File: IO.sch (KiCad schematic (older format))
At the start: 7 parts

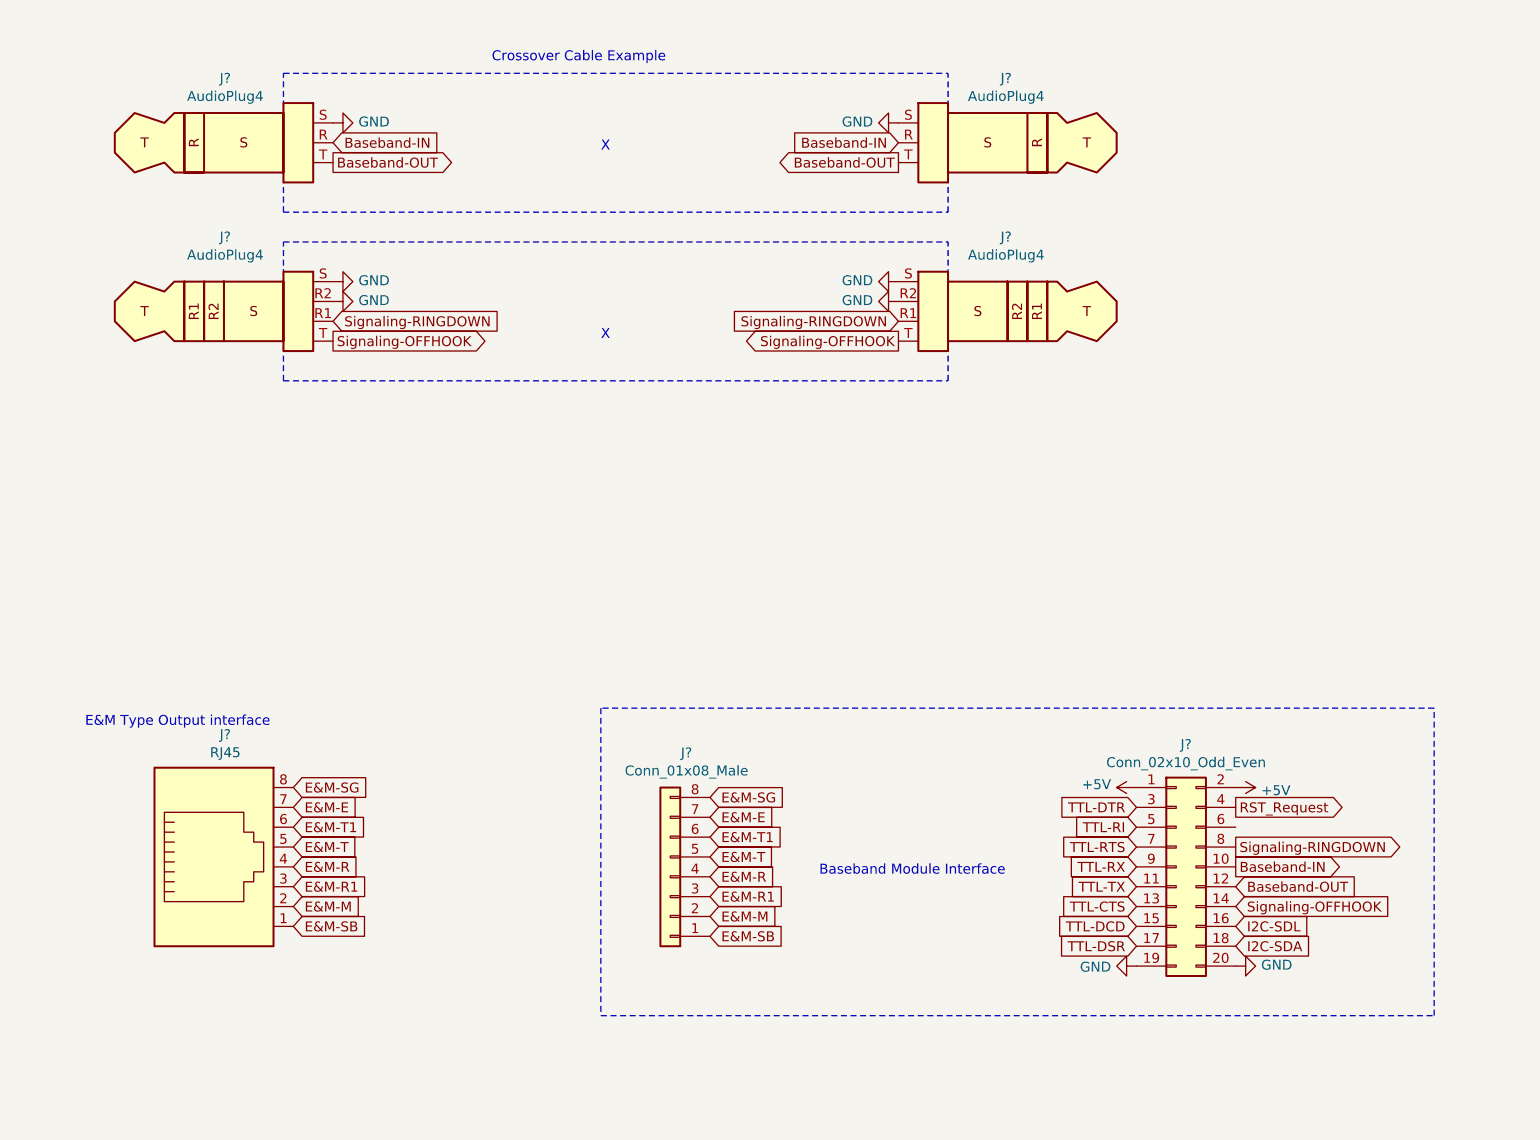
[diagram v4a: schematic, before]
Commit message: io interface updates
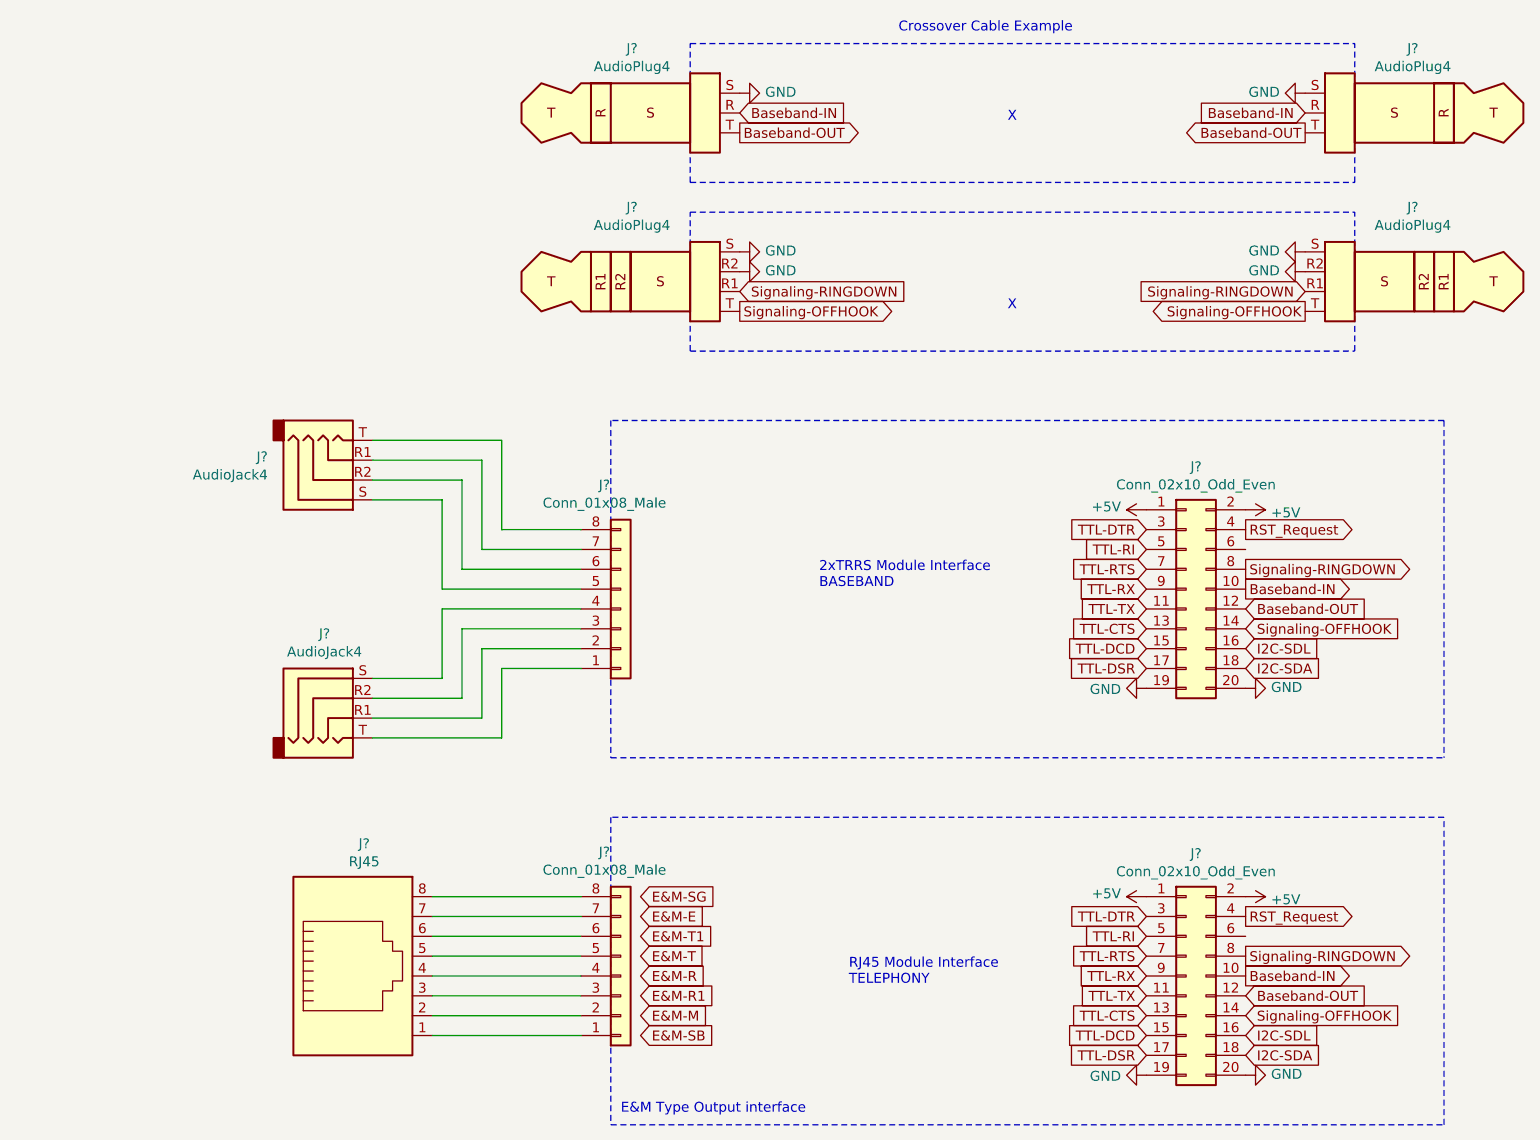
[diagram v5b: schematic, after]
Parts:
- added J?: Conn_01x08_Male, symbol Connector_Generic:Conn_01x08
- added J?: Conn_02x10_Odd_Even, symbol Connector_Generic:Conn_02x10_Odd_Even
- added J? (x2): AudioJack4, symbol Connector:AudioJack4
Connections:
- net +5V: now also J?.1 (Pin_1), J?.2 (Pin_2)
- net Baseband-IN: now also J?.10 (Pin_10)
- net Baseband-OUT: now also J?.12 (Pin_12)
- net E&M-E: no longer J?.7, J?.7 (Pin_7)
- net E&M-M: no longer J?.2, J?.2 (Pin_2)
- net E&M-R: no longer J?.4, J?.4 (Pin_4)
- net E&M-R1: no longer J?.3, J?.3 (Pin_3)
- net E&M-SB: no longer J?.1, J?.1 (Pin_1)
- net E&M-SG: no longer J?.8, J?.8 (Pin_8)
- net E&M-T: no longer J?.5, J?.5 (Pin_5)
- net E&M-T1: no longer J?.6, J?.6 (Pin_6)
- net GND: now also J?.19 (Pin_19), J?.20 (Pin_20)
- net I2C-SDA: now also J?.18 (Pin_18)
- net I2C-SDL: now also J?.16 (Pin_16)
- net RST_Request: now also J?.4 (Pin_4)
- net Signaling-OFFHOOK: now also J?.14 (Pin_14)
- net Signaling-RINGDOWN: now also J?.8 (Pin_8)
- net TTL-CTS: now also J?.13 (Pin_13)
- net TTL-DCD: now also J?.15 (Pin_15)
- net TTL-DSR: now also J?.17 (Pin_17)
- net TTL-DTR: now also J?.3 (Pin_3)
- net TTL-RI: now also J?.5 (Pin_5)
- net TTL-RTS: now also J?.7 (Pin_7)
- net TTL-RX: now also J?.9 (Pin_9)
- net TTL-TX: now also J?.11 (Pin_11)
- new net: J?.1, J?.1 (Pin_1)
- new net: J?.2, J?.2 (Pin_2)
- new net: J?.3, J?.3 (Pin_3)
- new net: J?.4, J?.4 (Pin_4)
- new net: J?.5, J?.5 (Pin_5)
- new net: J?.6, J?.6 (Pin_6)
- new net: J?.7, J?.7 (Pin_7)
- new net: J?.8, J?.8 (Pin_8)
- new net: J?.1 (Pin_1), J?.T
- new net: J?.2 (Pin_2), J?.R1
- new net: J?.3 (Pin_3), J?.R2
- new net: J?.4 (Pin_4), J?.S
- new net: J?.5 (Pin_5), J?.S
- new net: J?.6 (Pin_6), J?.R2
- new net: J?.7 (Pin_7), J?.R1
- new net: J?.8 (Pin_8), J?.T
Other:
- note added: "2xTRRS Module Interface\nBASEBAND"
- note added: "RJ45 Module Interface\nTELEPHONY"
- note removed: "Baseband Module Interface"
- moved on the sheet: J?

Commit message: updates
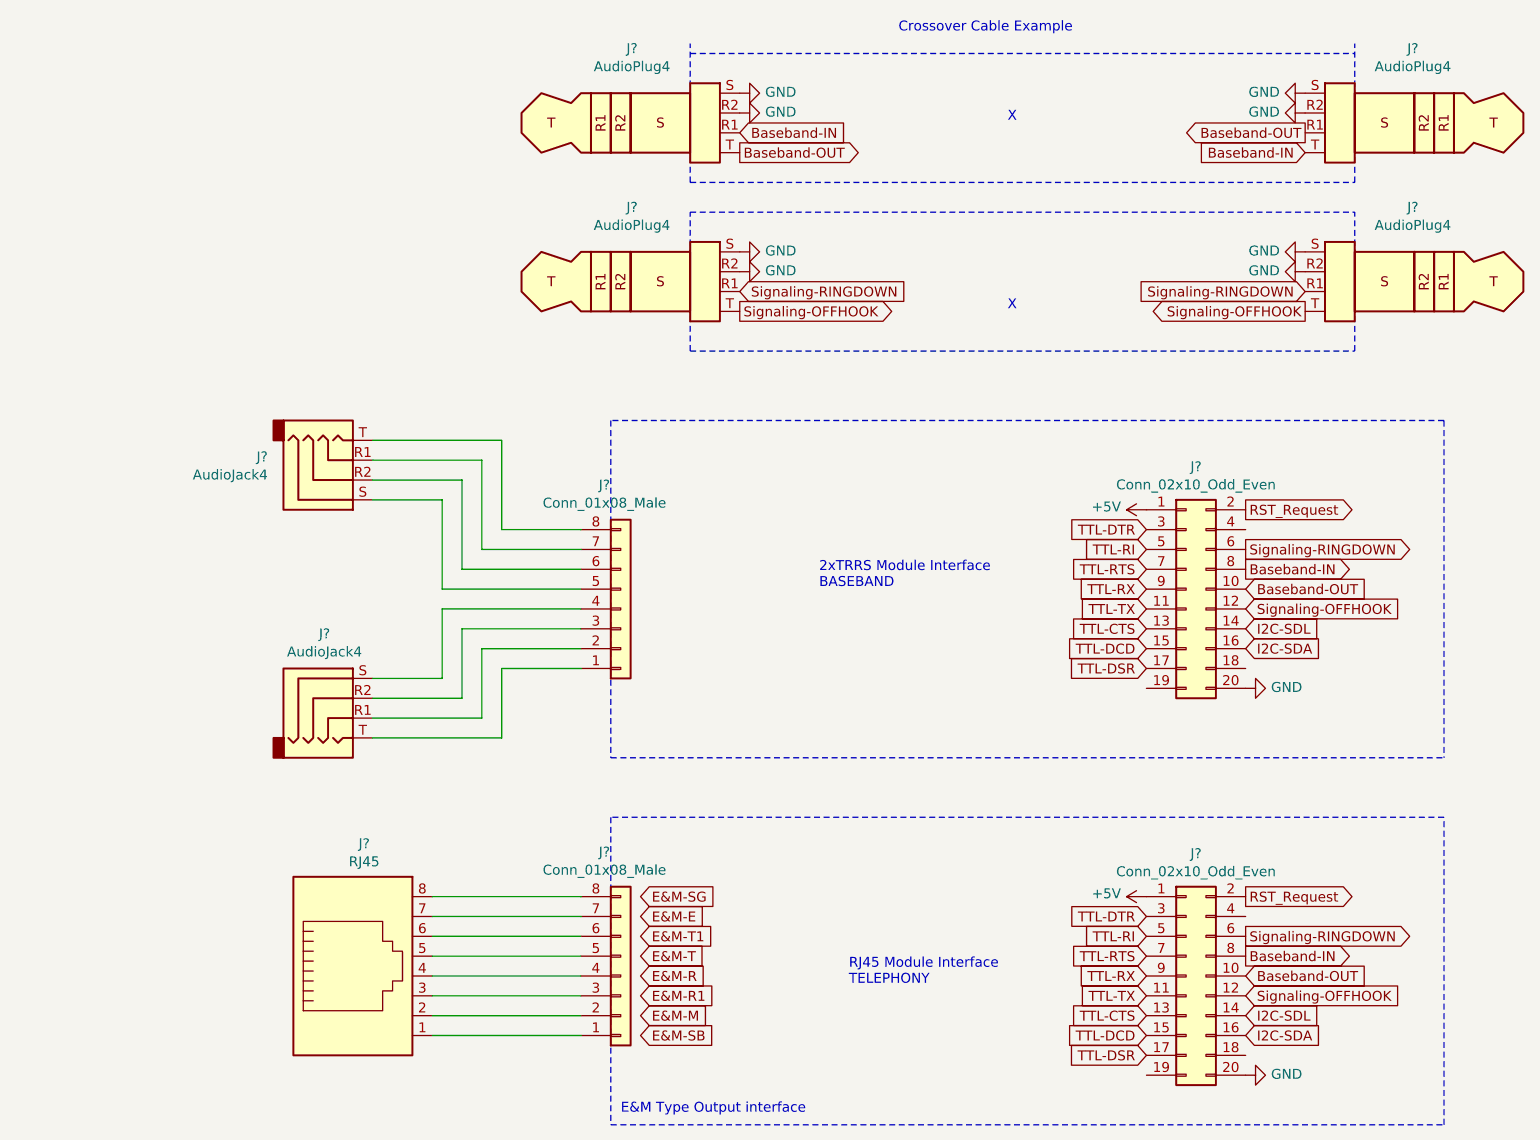
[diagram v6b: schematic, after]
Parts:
- removed J? (x2): AudioPlug4, symbol Connector:AudioPlug3
- added J? (x2): AudioPlug4, symbol Connector:AudioPlug4
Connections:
- net +5V: no longer J?.2 (Pin_2), J?.2 (Pin_2)
- net Baseband-IN: now also J?.8 (Pin_8), J?.8 (Pin_8), J?.R1, J?.T; no longer J?.10 (Pin_10), J?.10 (Pin_10)
- net Baseband-OUT: now also J?.10 (Pin_10), J?.10 (Pin_10), J?.R1, J?.T; no longer J?.12 (Pin_12), J?.12 (Pin_12)
- net GND: now also J?.R2, J?.R2, J?.S, J?.S; no longer J?.19 (Pin_19), J?.19 (Pin_19)
- net I2C-SDA: now also J?.16 (Pin_16), J?.16 (Pin_16); no longer J?.18 (Pin_18), J?.18 (Pin_18)
- net I2C-SDL: now also J?.14 (Pin_14), J?.14 (Pin_14); no longer J?.16 (Pin_16), J?.16 (Pin_16)
- net RST_Request: now also J?.2 (Pin_2), J?.2 (Pin_2); no longer J?.4 (Pin_4), J?.4 (Pin_4)
- net Signaling-OFFHOOK: now also J?.12 (Pin_12), J?.12 (Pin_12); no longer J?.14 (Pin_14), J?.14 (Pin_14)
- net Signaling-RINGDOWN: now also J?.6 (Pin_6), J?.6 (Pin_6); no longer J?.8 (Pin_8), J?.8 (Pin_8)
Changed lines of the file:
@@
-$EndComp
-$Comp
-L power:GND #PWR?
-U 1 1 60EA1224
-P 6550 6100
-AR Path="/60EA1224" Ref="#PWR?"  Part="1"
-AR Path="/60E9D9E5/60EA1224" Ref="#PWR?"  Part="1"
-F 0 "#PWR?" H 6550 5850 50  0001 C CNN
-F 1 "GND" V 6555 5972 50  0000 R CNN
-F 2 "" H 6550 6100 50  0001 C CNN
-F 3 "" H 6550 6100 50  0001 C CNN
-	1    6550 6100
-	0    1    1    0
-$EndComp
-$Comp
-L power:+5V #PWR?
-U 1 1 60EA122A
-P 7050 5200
-AR Path="/60EA122A" Ref="#PWR?"  Part="1"
-AR Path="/60E9D9E5/60EA122A" Ref="#PWR?"  Part="1"
-F 0 "#PWR?" H 7050 5050 50  0001 C CNN
-F 1 "+5V" V 7065 5328 50  0000 L CNN
-F 2 "" H 7050 5200 50  0001 C CNN
-F 3 "" H 7050 5200 50  0001 C CNN
-	1    7050 5200
-	0    1    1    0
 $EndComp
 $Comp
@@
 Text Notes 4900 3650 0    50   ~ 0
 2xTRRS Module Interface\nBASEBAND
-Text GLabel 7050 5300 2    50   Output ~ 0
+Text GLabel 7050 5200 2    50   Output ~ 0
 RST_Request
-$Comp
-L Connector:AudioPlug3 J?
-U 1 1 60EB32CF
-P 3900 1250
-AR Path="/60EB32CF" Ref="J?"  Part="1"
-AR Path="/60E9D9E5/60EB32CF" Ref="J?"  Part="1"
-F 0 "J?" H 3957 1575 50  0000 C CNN
-F 1 "AudioPlug4" H 3957 1484 50  0000 C CNN
-F 2 "" H 4250 1150 50  0001 C CNN
-F 3 "~" H 4250 1150 50  0001 C CNN
-	1    3900 1250
-	1    0    0    -1
-$EndComp
 $Comp
 L power:GND #PWR?
@@
 	0    -1   -1   0
 $EndComp
-Text GLabel 4500 1350 2    50   Output ~ 0
+Text GLabel 4500 1450 2    50   Output ~ 0
 Baseband-OUT
 Text GLabel 4500 2250 2    50   Output ~ 0
@@
 Wire Notes Line
 	8050 6350 8050 4800
-$Comp
-L Connector:AudioPlug3 J?
-U 1 1 60EE43AB
-P 7950 1250
-AR Path="/60EE43AB" Ref="J?"  Part="1"
-AR Path="/60E9D9E5/60EE43AB" Ref="J?"  Part="1"
-F 0 "J?" H 8007 1575 50  0000 C CNN
-F 1 "AudioPlug4" H 8007 1484 50  0000 C CNN
-F 2 "" H 8300 1150 50  0001 C CNN
-F 3 "~" H 8300 1150 50  0001 C CNN
-	1    7950 1250
-	-1   0    0    -1
-$EndComp
 $Comp
 L power:GND #PWR?
@@
 	0    1    -1   0
 $EndComp
-Text GLabel 7350 1250 0    50   Input ~ 0
+Text GLabel 7350 1450 0    50   Input ~ 0
 Baseband-IN
 Text GLabel 7350 2150 0    50   Input ~ 0
@@
 Text Notes 5300 850  0    50   ~ 0
 Crossover Cable Example
-Text GLabel 7050 6000 2    50   Input ~ 0
+Text GLabel 7050 5900 2    50   Input ~ 0
 I2C-SDA
-Text GLabel 7050 5900 2    50   Input ~ 0
+Text GLabel 7050 5800 2    50   Input ~ 0
 I2C-SDL
 $Comp
@@
 	0    -1   -1   0
 $EndComp
+Text GLabel 7050 5400 2    50   Output ~ 0
+Signaling-RINGDOWN
+Text GLabel 7050 5700 2    50   Input ~ 0
+Signaling-OFFHOOK
+Text GLabel 7050 5600 2    50   Input ~ 0
+Baseband-OUT
 Text GLabel 7050 5500 2    50   Output ~ 0
-Signaling-RINGDOWN
-Text GLabel 7050 5800 2    50   Input ~ 0
-Signaling-OFFHOOK
-Text GLabel 7050 5700 2    50   Input ~ 0
-Baseband-OUT
-Text GLabel 7050 5600 2    50   Output ~ 0
 Baseband-IN
 $Comp
@@
 	0    1    -1   0
 $EndComp
-Text GLabel 4500 1250 2    50   Input ~ 0
+Text GLabel 4500 1350 2    50   Input ~ 0
 Baseband-IN
 Text GLabel 4500 2150 2    50   Input ~ 0
@@
 	4250 2450 7600 2450
 Wire Notes Line
-	4250 900  7600 900
+	4250 950  7600 950
 Wire Notes Line
 	4250 1600 7600 1600
@@
 	1    3900 3750
 	1    0    0    1
-$EndComp
-$Comp
-L power:GND #PWR?
-U 1 1 60F6E687
-P 6550 4150
-AR Path="/60F6E687" Ref="#PWR?"  Part="1"
-AR Path="/60E9D9E5/60F6E687" Ref="#PWR?"  Part="1"
-F 0 "#PWR?" H 6550 3900 50  0001 C CNN
-F 1 "GND" V 6555 4022 50  0000 R CNN
-F 2 "" H 6550 4150 50  0001 C CNN
-F 3 "" H 6550 4150 50  0001 C CNN
-	1    6550 4150
-	0    1    1    0
-$EndComp
-$Comp
-L power:+5V #PWR?
-U 1 1 60F6E691
-P 7050 3250
-AR Path="/60F6E691" Ref="#PWR?"  Part="1"
-AR Path="/60E9D9E5/60F6E691" Ref="#PWR?"  Part="1"
-F 0 "#PWR?" H 7050 3100 50  0001 C CNN
-F 1 "+5V" V 7065 3378 50  0000 L CNN
-F 2 "" H 7050 3250 50  0001 C CNN
-F 3 "" H 7050 3250 50  0001 C CNN
-	1    7050 3250
-	0    1    1    0
 $EndComp
 $Comp
@@
 Text Notes 5050 5650 0    50   ~ 0
 RJ45 Module Interface\nTELEPHONY
-Text GLabel 7050 3350 2    50   Output ~ 0
+Text GLabel 7050 3250 2    50   Output ~ 0
 RST_Request
 Wire Notes Line
 	8050 2800 3850 2800
-Text GLabel 7050 4050 2    50   Input ~ 0
+Text GLabel 7050 3950 2    50   Input ~ 0
 I2C-SDA
-Text GLabel 7050 3950 2    50   Input ~ 0
+Text GLabel 7050 3850 2    50   Input ~ 0
 I2C-SDL
 $Comp
@@
 	0    -1   -1   0
 $EndComp
+Text GLabel 7050 3450 2    50   Output ~ 0
+Signaling-RINGDOWN
+Text GLabel 7050 3750 2    50   Input ~ 0
+Signaling-OFFHOOK
+Text GLabel 7050 3650 2    50   Input ~ 0
+Baseband-OUT
 Text GLabel 7050 3550 2    50   Output ~ 0
-Signaling-RINGDOWN
-Text GLabel 7050 3850 2    50   Input ~ 0
-Signaling-OFFHOOK
-Text GLabel 7050 3750 2    50   Input ~ 0
-Baseband-OUT
-Text GLabel 7050 3650 2    50   Output ~ 0
 Baseband-IN
 $Comp
@@
 Wire Notes Line
 	8050 2800 8050 4500
+$Comp
+L Connector:AudioPlug4 J?
+U 1 1 60FDB7A8
+P 3900 1250
+AR Path="/60FDB7A8" Ref="J?"  Part="1"
+AR Path="/60E9D9E5/60FDB7A8" Ref="J?"  Part="1"
+F 0 "J?" H 3957 1575 50  0000 C CNN
+F 1 "AudioPlug4" H 3957 1484 50  0000 C CNN
+F 2 "" H 4250 1150 50  0001 C CNN
+F 3 "~" H 4250 1150 50  0001 C CNN
+	1    3900 1250
+	1    0    0    -1
+$EndComp
+$Comp
+L Connector:AudioPlug4 J?
+U 1 1 60FDC067
+P 7950 1250
+AR Path="/60FDC067" Ref="J?"  Part="1"
+AR Path="/60E9D9E5/60FDC067" Ref="J?"  Part="1"
+F 0 "J?" H 8007 1575 50  0000 C CNN
+F 1 "AudioPlug4" H 8007 1484 50  0000 C CNN
+F 2 "" H 8300 1150 50  0001 C CNN
+F 3 "~" H 8300 1150 50  0001 C CNN
+	1    7950 1250
+	-1   0    0    -1
+$EndComp
+$Comp
+L power:GND #PWR?
+U 1 1 60FE2765
+P 4500 1250
+AR Path="/60FE2765" Ref="#PWR?"  Part="1"
+AR Path="/60E9D9E5/60FE2765" Ref="#PWR?"  Part="1"
+F 0 "#PWR?" H 4500 1000 50  0001 C CNN
+F 1 "GND" V 4505 1122 50  0000 R CNN
+F 2 "" H 4500 1250 50  0001 C CNN
+F 3 "" H 4500 1250 50  0001 C CNN
+	1    4500 1250
+	0    -1   -1   0
+$EndComp
+$Comp
+L power:GND #PWR?
+U 1 1 60FE2987
+P 7350 1250
+AR Path="/60FE2987" Ref="#PWR?"  Part="1"
+AR Path="/60E9D9E5/60FE2987" Ref="#PWR?"  Part="1"
+F 0 "#PWR?" H 7350 1000 50  0001 C CNN
+F 1 "GND" V 7355 1122 50  0000 R CNN
+F 2 "" H 7350 1250 50  0001 C CNN
+F 3 "" H 7350 1250 50  0001 C CNN
+	1    7350 1250
+	0    1    -1   0
+$EndComp
 $EndSCHEMATC

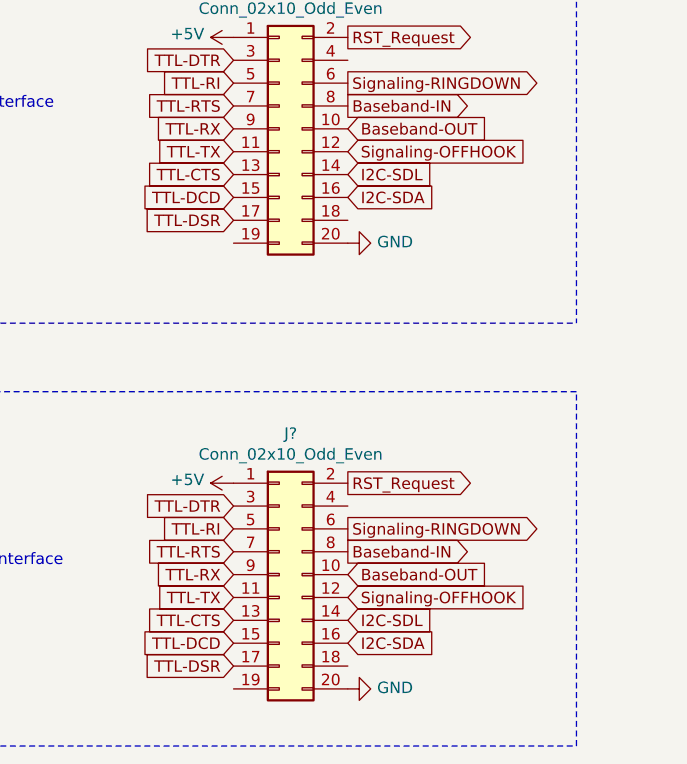
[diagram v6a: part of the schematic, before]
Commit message: general updates
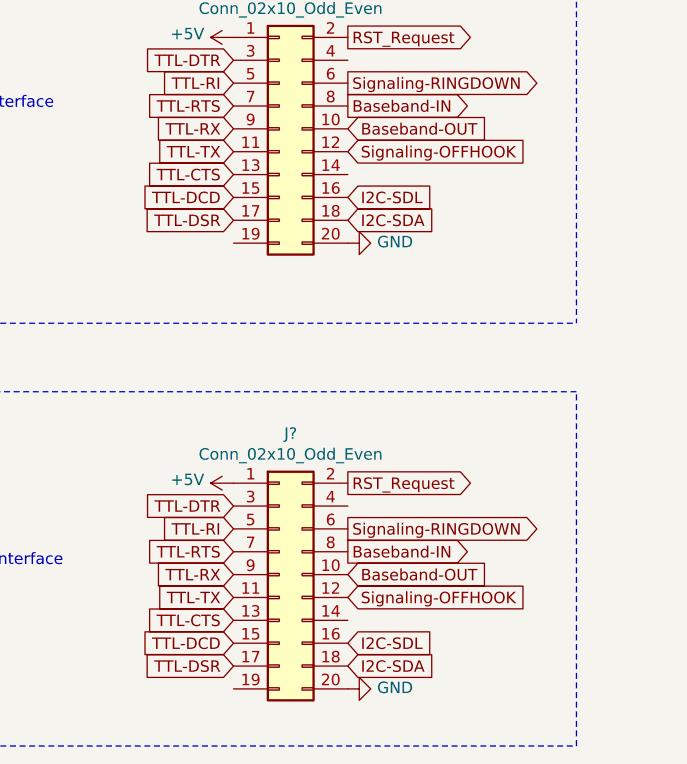
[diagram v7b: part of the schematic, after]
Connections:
- net I2C-SDA: now also J?.18 (Pin_18), J?.18 (Pin_18); no longer J?.16 (Pin_16), J?.16 (Pin_16)
- net I2C-SDL: now also J?.16 (Pin_16), J?.16 (Pin_16); no longer J?.14 (Pin_14), J?.14 (Pin_14)
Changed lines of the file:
@@
 $Descr A4 11693 8268
 encoding utf-8
-Sheet 6 11
+Sheet 6 12
 Title "300 Baud Audio FSK Modem "
 Date "2021-07-08"
@@
 Text Notes 5300 850  0    50   ~ 0
 Crossover Cable Example
+Text GLabel 7050 6000 2    50   Input ~ 0
+I2C-SDA
 Text GLabel 7050 5900 2    50   Input ~ 0
-I2C-SDA
-Text GLabel 7050 5800 2    50   Input ~ 0
 I2C-SDL
 $Comp
@@
 Wire Notes Line
 	8050 2800 3850 2800
+Text GLabel 7050 4050 2    50   Input ~ 0
+I2C-SDA
 Text GLabel 7050 3950 2    50   Input ~ 0
-I2C-SDA
-Text GLabel 7050 3850 2    50   Input ~ 0
 I2C-SDL
 $Comp
